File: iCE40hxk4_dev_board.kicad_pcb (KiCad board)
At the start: 4 copper layers, 67 x 161.8 mm, 383 parts, among them J1001 Testpoint, J1002 Testpoint, J1003 Testpoint, J1004 Testpoint, J1005 USB_EXT, J101 CONN_01X02, J102 Jack Estereo, J103 CONN_COAXIAL, J104 CONN_COAXIAL, J105 MountingHole, J106 MountingHole, J107 MountingHole, J108 MountingHole, J1101 CONN_01X25, J202 USB_OTG, J401 Testpoint, J402 Testpoint, J403 Testpoint, J404 Testpoint, J405 Testpoint, J406 Testpoint, J501 Testpoint, J502 Testpoint, J601 CONN_01X02, J602 CONN_01X02, J603 Testpoint, J604 Testpoint, J605 Testpoint, J701 Testpoint, J702 Testpoint, J705 Testpoint, J706 Testpoint, J801 Testpoint, J802 Testpoint, J803 Testpoint, J804 Testpoint, J805 Testpoint, J806 Testpoint, J807 Testpoint, J808 Testpoint, J809 Testpoint, J810 Testpoint, SW1101 SW_Push, U1001 ADC1175, U1002 ADC1175, U1101 MIC7300, U1102 MIC7300, U1103 MCP4716, U1104 MCP4716, U1105 MIC7300, U1106 MIC7300, U201 MIC2005A-2YM5, U203 93LC56BT-I/OT, U204 MIC5355-S4YMME, U205 FT2232H, U301 iCE40-HX4K-TQ144, U302 FLASH 2Mb, U501 AS4C1M16S-7TCN, U701 CPC1017N, U702 CPC1017N, U703 CD4051BM96, U704 CD4051BM96, U801 CD4051BM96, U802 CD4051BM96, U803 CLC4007, U901 LM2776DBVR, U902 TCR2EF13,LM, U903 MIC5270

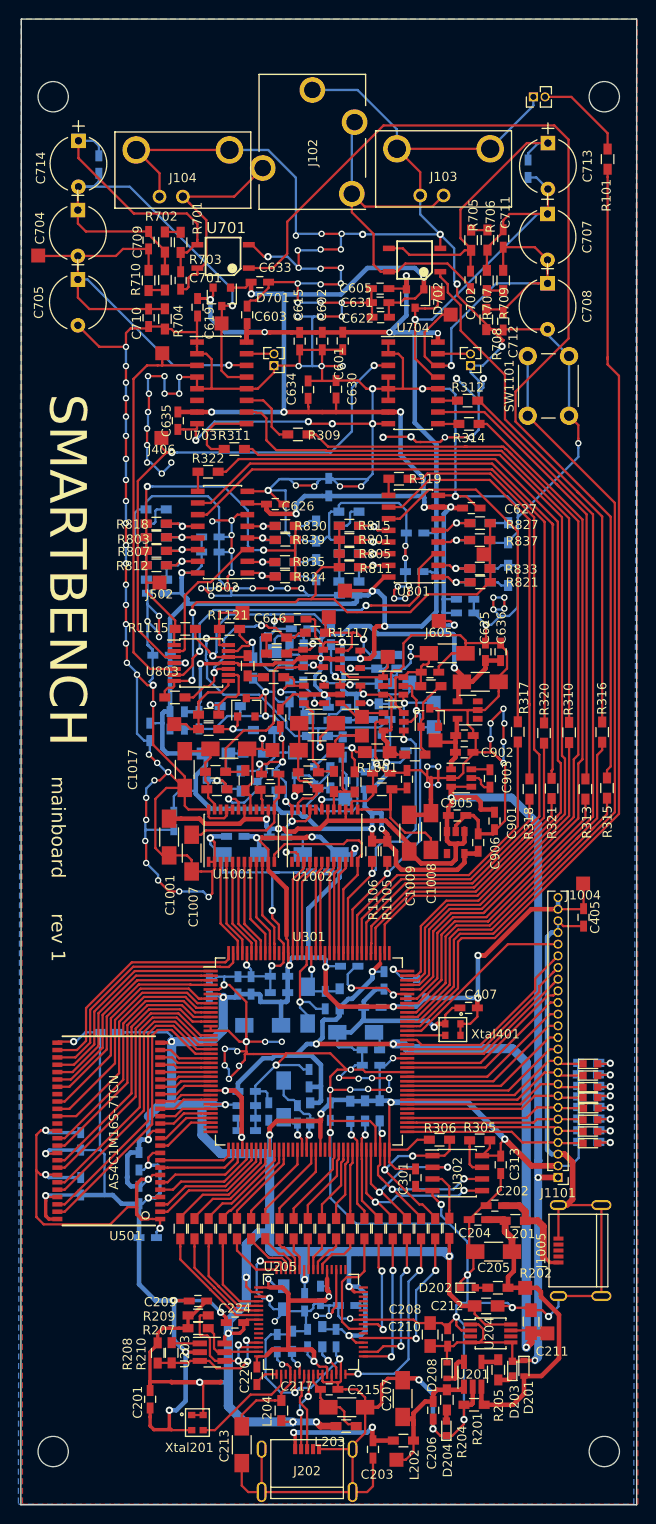
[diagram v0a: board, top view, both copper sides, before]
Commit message: Fab files
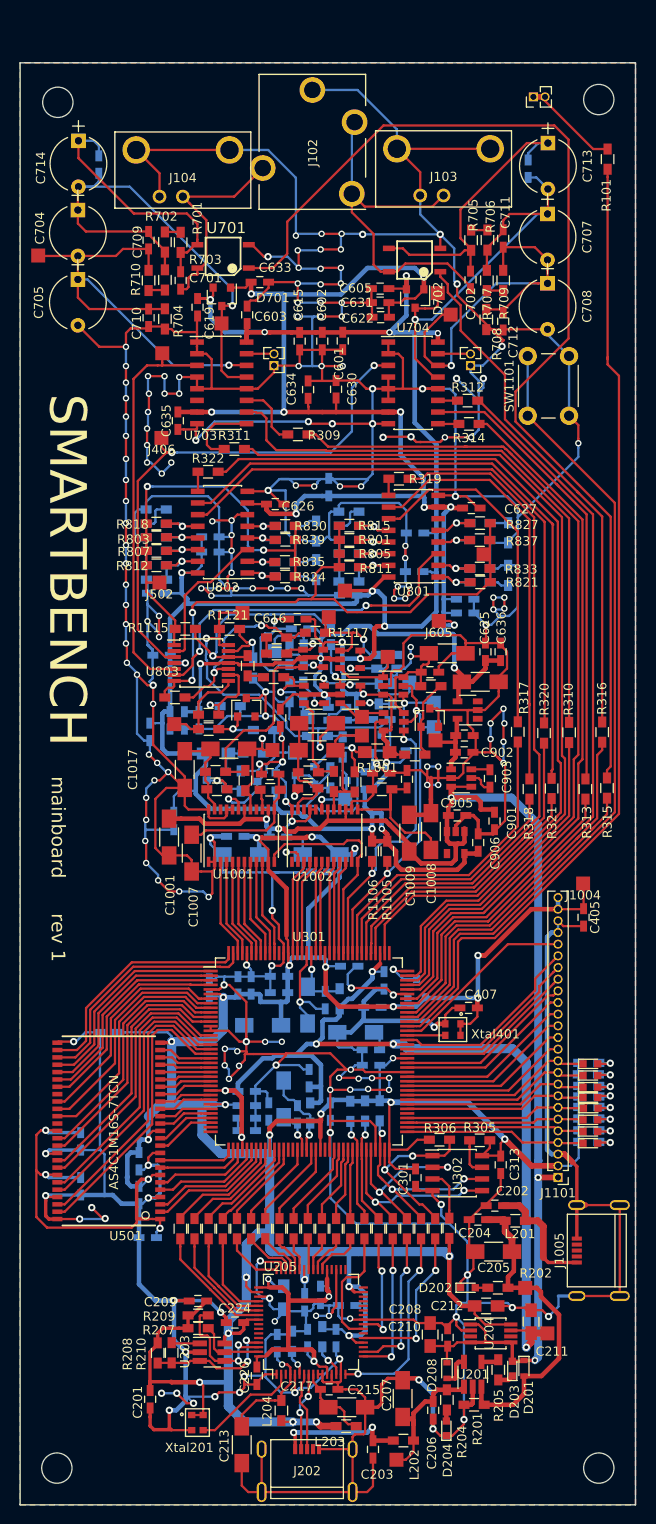
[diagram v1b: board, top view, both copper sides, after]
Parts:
- moved J1005 2.00 mm to (149.4, 163.1)
- moved J106 1.90 mm to (150.9, 188.8)
- moved J105 1.85 mm to (90.9, 188.8)
- moved J107 0.79 mm to (91.4, 37.8)
- moved J108 0.67 mm to (150.7, 37.9)
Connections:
- J1005 pad 2: Net-(J1005-Pad2) -> (no net)
- J1005 pad 3: Net-(J1005-Pad3) -> (no net)
- J1005 pad 4: Net-(J1005-Pad4) -> (no net)
- J101 pad 1: GND -> Net-(J101-Pad1)
- J101 pad 2: Net-(J101-Pad2) -> Net-(J101-Pad1)
- J202 pad 4: Net-(J202-Pad4) -> (no net)
- R101 pad 2: Net-(J101-Pad2) -> Net-(J101-Pad1)
- U1001 pad 16: Net-(U1001-Pad16) -> (no net)
- U1001 pad 22: Net-(U1001-Pad22) -> (no net)
- U1002 pad 16: Net-(U1002-Pad16) -> (no net)
- U1002 pad 22: Net-(U1002-Pad22) -> (no net)
- U205 pad 19: Net-(U205-Pad19) -> (no net)
- U205 pad 22: Net-(U205-Pad22) -> (no net)
- U205 pad 26: Net-(U205-Pad26) -> (no net)
- U205 pad 27: Net-(U205-Pad27) -> (no net)
- U205 pad 28: Net-(U205-Pad28) -> (no net)
- U205 pad 29: Net-(U205-Pad29) -> (no net)
- U205 pad 3: Net-(U205-Pad3) -> (no net)
- U205 pad 30: Net-(U205-Pad30) -> (no net)
- U205 pad 32: Net-(U205-Pad32) -> (no net)
- U205 pad 33: Net-(U205-Pad33) -> (no net)
- U205 pad 34: Net-(U205-Pad34) -> (no net)
- U205 pad 36: Net-(U205-Pad36) -> (no net)
- U205 pad 57: Net-(U205-Pad57) -> (no net)
- U205 pad 58: Net-(U205-Pad58) -> (no net)
- U205 pad 59: Net-(U205-Pad59) -> (no net)
- U205 pad 60: Net-(U205-Pad60) -> (no net)
- U301 pad 109: Net-(U301-Pad109) -> (no net)
- U301 pad 133: Net-(U301-Pad133) -> (no net)
- U301 pad 35: Net-(U301-Pad35) -> (no net)
- U301 pad 36: Net-(U301-Pad36) -> (no net)
- U301 pad 50: Net-(U301-Pad50) -> (no net)
- U301 pad 51: Net-(U301-Pad51) -> (no net)
- U301 pad 58: Net-(U301-Pad58) -> (no net)
- U301 pad 77: Net-(U301-Pad77) -> (no net)
- U501 pad 33: Net-(U501-Pad33) -> (no net)
- U501 pad 37: Net-(U501-Pad37) -> (no net)
- U902 pad 4: Net-(U902-Pad4) -> (no net)
- U903 pad 1: Net-(U903-Pad1) -> (no net)
- U903 pad 3: Net-(U903-Pad3) -> (no net)
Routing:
- net GND: track 1532.8 -> 1551.8 mm, vias 188 -> 197
- net Net-(J101-Pad1): track 0.00 -> 10.7 mm
- net Net-(J101-Pad2): track 10.2 -> 0.00 mm
- net +3V3: track 507.6 -> 504.3 mm
- net Net-(C202-Pad1): track 11.1 -> 13.3 mm
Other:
- board size 67 x 161.8 mm -> 67 x 157 mm
